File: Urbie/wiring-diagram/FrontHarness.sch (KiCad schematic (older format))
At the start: 19 parts

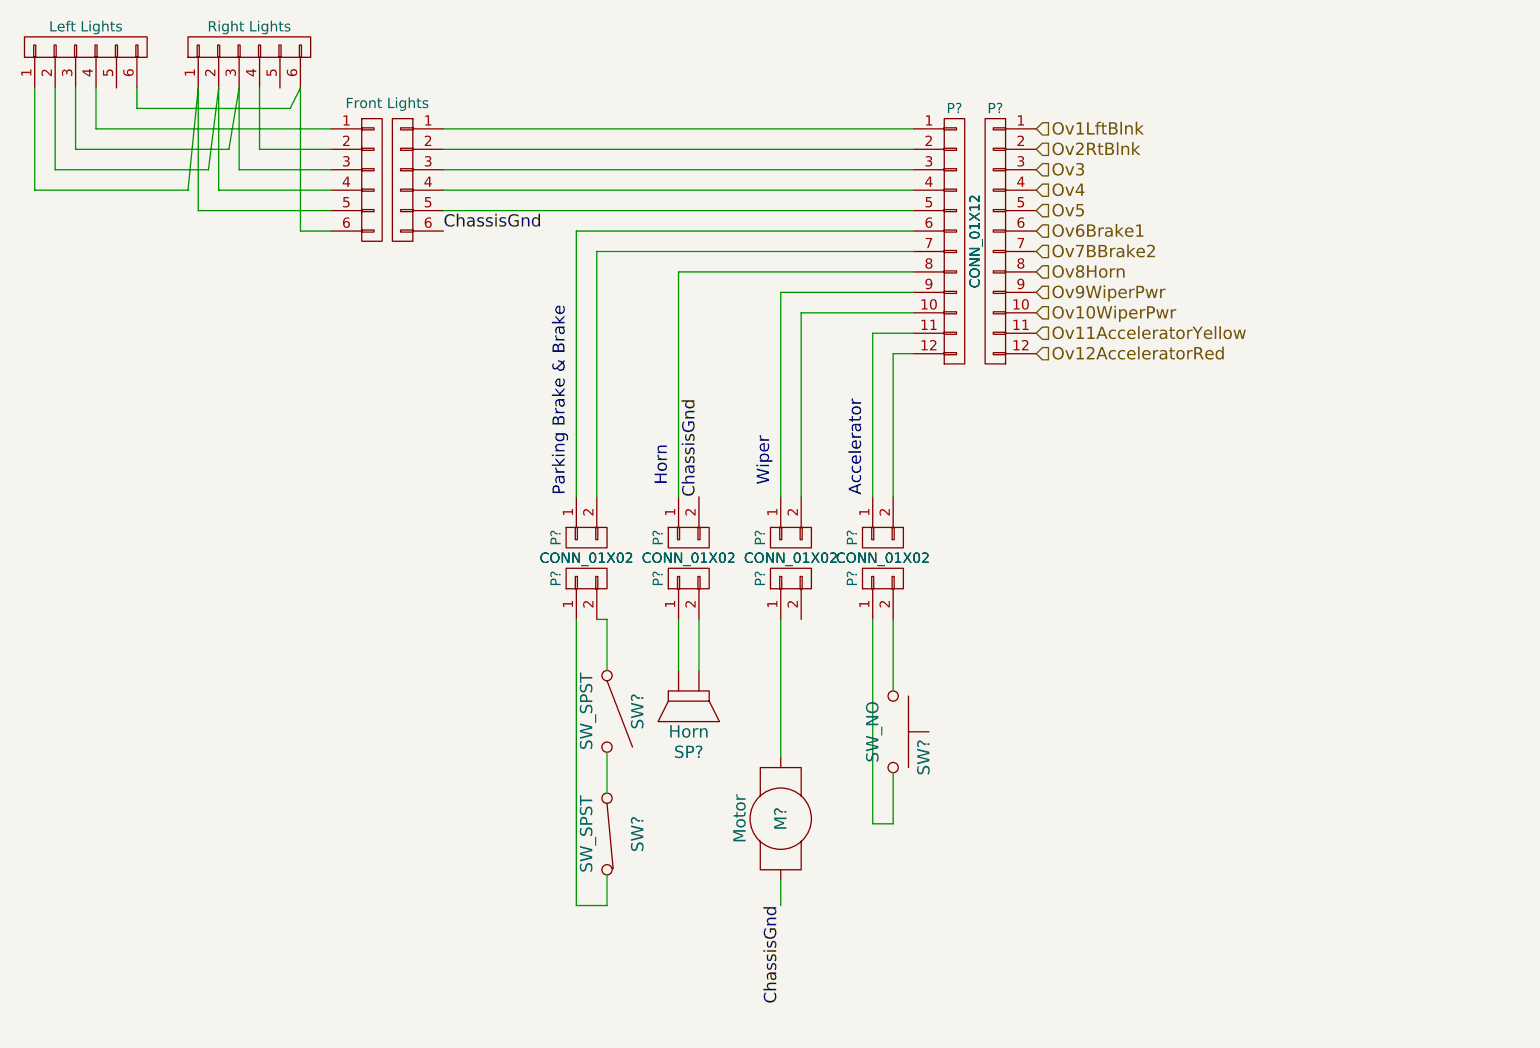
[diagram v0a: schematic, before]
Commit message: updated 1593BB-box footprint
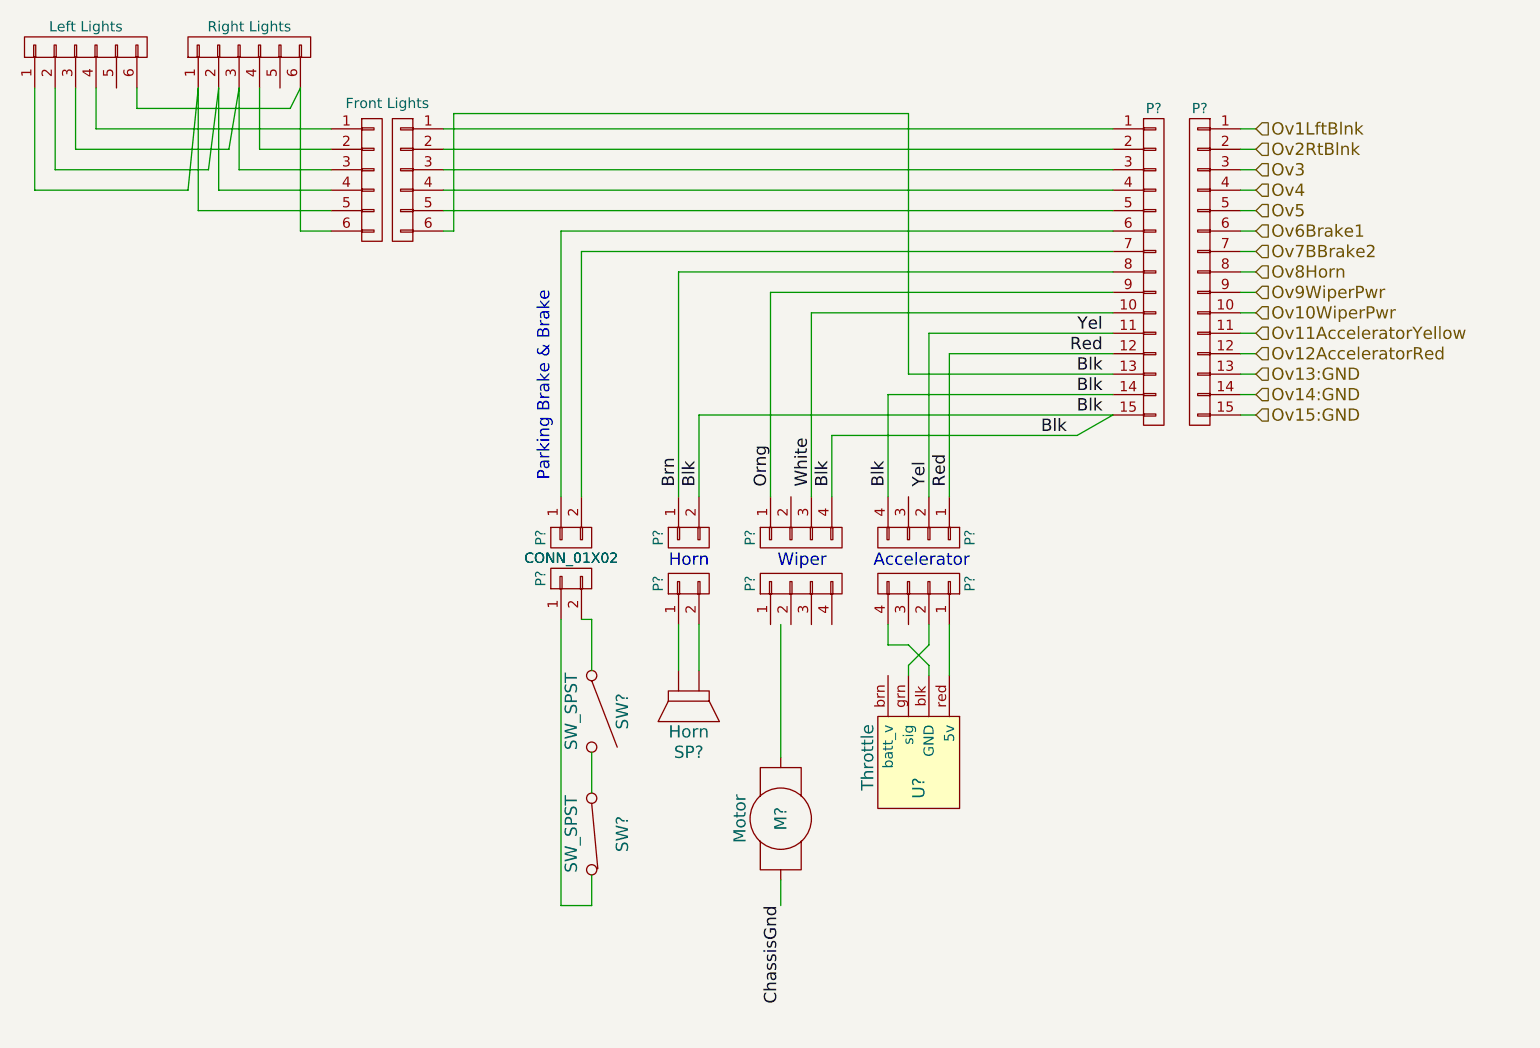
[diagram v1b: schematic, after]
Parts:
- removed P? (x2): CONN_01X12, symbol CONN_01X12
- removed P? (x4): CONN_01X02, symbol CONN_01X02
- removed SW?: SW_NO, symbol SW_NO
- added P? (x2): CONN_01X15, symbol CONN_01X15
- added P? (x4): CONN_01X04, symbol CONN_01X04
- added U?: Throttle, symbol Throttle
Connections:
- net ChassisGnd: no longer P?.2 (P2), P?.6 (P6)
- net Ov10WiperPwr: now also P?.10 (P10)
- net Ov11AcceleratorYellow: now also P?.11 (P11)
- net Ov12AcceleratorRed: now also P?.12 (P12)
- net Ov1LftBlnk: now also P?.1 (P1)
- net Ov2RtBlnk: now also P?.2 (P2)
- net Ov3: now also P?.3 (P3)
- net Ov4: now also P?.4 (P4)
- net Ov5: now also P?.5 (P5)
- net Ov6Brake1: now also P?.6 (P6)
- net Ov7BBrake2: now also P?.7 (P7)
- net Ov8Horn: now also P?.8 (P8)
- net Ov9WiperPwr: now also P?.9 (P9)
- net at P?.1 (P1): now also P?.1 (P1)
- net at P?.2 (P2): now also P?.2 (P2)
- net at P?.3 (P3): now also P?.3 (P3)
- net at P?.4 (P4): now also P?.4 (P4)
- net at P?.5 (P5): now also P?.5 (P5)
- net at P?.1 (P1): now also P?.6 (P6)
- net at P?.2 (P2): now also P?.7 (P7)
- net Brn: now reaches P?.1 (P1)
- net Brn: now also P?.8 (P8)
- new net: P?.4 (P4), U?.blk (GND)
- new net: P?.2 (P2), U?.grn (sig)
- new net: P?.1 (P1), U?.red (5v)
- new net Blk: P?.13 (P13), P?.14 (P14), P?.15 (P15), P?.2 (P2), P?.4 (P4), P?.4 (P4), P?.6 (P6)
- new net Orng: P?.1 (P1), P?.9 (P9)
- new net Ov13:GND: P?.13 (P13)
- new net Ov14:GND: P?.14 (P14)
- new net Ov15:GND: P?.15 (P15)
- new net Red: P?.1 (P1), P?.12 (P12)
- new net White: P?.10 (P10), P?.3 (P3)
- new net Yel: P?.11 (P11), P?.2 (P2)
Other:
- moved on the sheet: P?, SW?
